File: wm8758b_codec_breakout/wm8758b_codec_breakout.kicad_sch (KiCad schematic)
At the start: 19 parts, among them J1 Conn_01x12, J101 AudioJack3, J102 AudioJack3, J2 Conn_01x12, U1 WM8758B

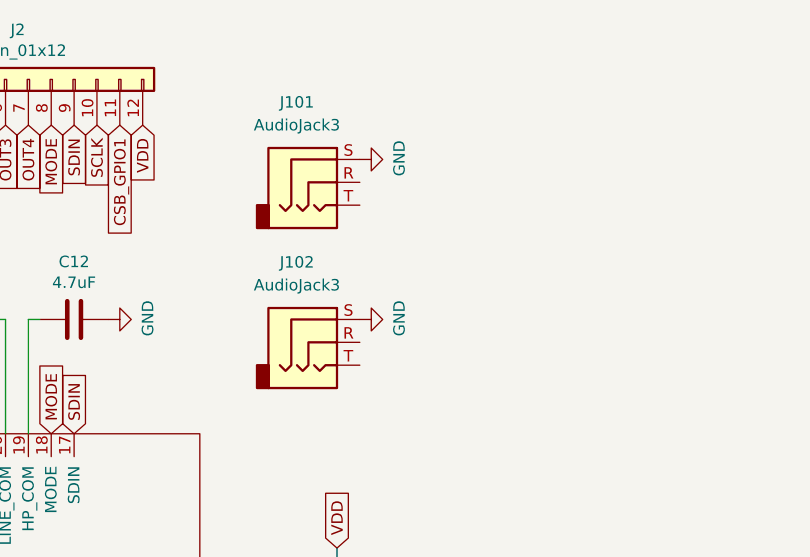
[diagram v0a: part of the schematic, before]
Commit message: WIP
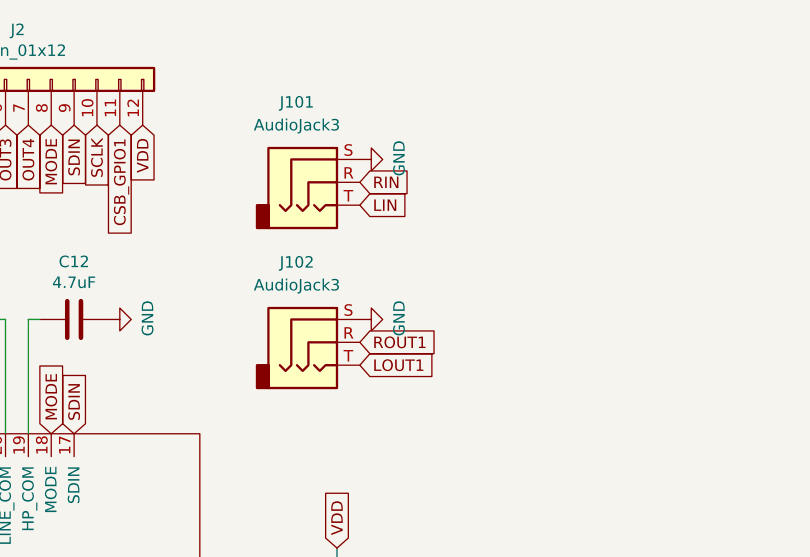
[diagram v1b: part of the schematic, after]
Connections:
- net LIN: now also J101.T
- net LOUT1: now also J102.T
- net RIN: now also J101.R
- net ROUT1: now also J102.R
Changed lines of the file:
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@@
+    )
+  )
+  (global_label "ROUT1" (shape input) (at 186.69 59.69 0) (fields_autoplaced)
+    (effects (font (size 1.27 1.27)) (justify left))
+    (property "Intersheet References" "${INTERSHEET_REFS}" (id 0) (at 309.88 156.21 0)
+      (effects (font (size 1.27 1.27)) hide)
     )
   )
@@
     )
   )
+  (global_label "RIN" (shape input) (at 186.69 41.91 0) (fields_autoplaced)
+    (effects (font (size 1.27 1.27)) (justify left))
+    (property "Intersheet References" "${INTERSHEET_REFS}" (id 0) (at 11.43 -88.9 0)
+      (effects (font (size 1.27 1.27)) hide)
+    )
+  )
   (global_label "RIP" (shape input) (at 175.26 140.97 0) (fields_autoplaced)
     (effects (font (size 1.27 1.27)) (justify left))
@@
     )
   )
+  (global_label "LOUT1" (shape input) (at 186.69 62.23 0) (fields_autoplaced)
+    (effects (font (size 1.27 1.27)) (justify left))
+    (property "Intersheet References" "${INTERSHEET_REFS}" (id 0) (at 309.88 161.29 0)
+      (effects (font (size 1.27 1.27)) hide)
+    )
+  )
   (global_label "OUT3" (shape input) (at 147.32 35.56 270) (fields_autoplaced)
     (effects (font (size 1.27 1.27)) (justify right))
@@
       (effects (font (size 1.27 1.27)) hide)
     )
+  )
+  (global_label "LIN" (shape input) (at 186.69 44.45 0) (fields_autoplaced)
+    (effects (font (size 1.27 1.27)) (justify left))
+    (property "Intersheet References" "${INTERSHEET_REFS}" (id 0) (at 300.99 187.96 0)
+      (effects (font (size 1.27 1.27)) hide)
+    )

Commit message: final touches + v1 jlcpcb fab files
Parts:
- J101, J102: LCSC Part (none) -> C707224; MSCS Part C707224 -> (none)
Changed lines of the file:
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@@
       (effects (font (size 1.27 1.27)) hide)
     )
-    (property "MSCS Part" "C707224" (id 4) (at 181.61 59.69 0)
+    (property "LCSC Part" "C707224" (id 4) (at 181.61 59.69 0)
       (effects (font (size 1.27 1.27)) hide)
     )
@@
       (effects (font (size 1.27 1.27)) hide)
     )
-    (property "MSCS Part" "C707224" (id 4) (at 181.61 41.91 0)
+    (property "LCSC Part" "C707224" (id 4) (at 181.61 41.91 0)
       (effects (font (size 1.27 1.27)) hide)
     )
